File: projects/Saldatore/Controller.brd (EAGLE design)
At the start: 50.8 x 33 mm, 20 parts, among them U1 ATTINY85-P

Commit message: in lavoro saldatore.
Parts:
- R4: value 47-2W -> 120-5W
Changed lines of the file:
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@@
 <drawing>
 <settings>
-<setting alwaysvectorfont="yes"/>
+<setting alwaysvectorfont="no"/>
 <setting verticaltext="up"/>
 </settings>
@@
 <attribute name="VALUE" x="32.29" y="22.99" size="1.27" layer="27" rot="R90"/>
 </element>
-<element name="R4" library="rcl" library_urn="urn:adsk.eagle:library:334" package="0204/7" package3d_urn="urn:adsk.eagle:package:23498/2" value="47-2W" x="36.83" y="44.45" smashed="yes" rot="R270">
+<element name="R4" library="rcl" library_urn="urn:adsk.eagle:library:334" package="0204/7" package3d_urn="urn:adsk.eagle:package:23498/2" value="120-5W" x="36.83" y="44.45" smashed="yes" rot="R270">
 <attribute name="NAME" x="38.1254" y="46.99" size="0.9906" layer="25" ratio="10" rot="R270"/>
 <attribute name="POPULARITY" value="79" x="-8.89" y="6.35" size="1.778" layer="27" rot="R270" display="off"/>

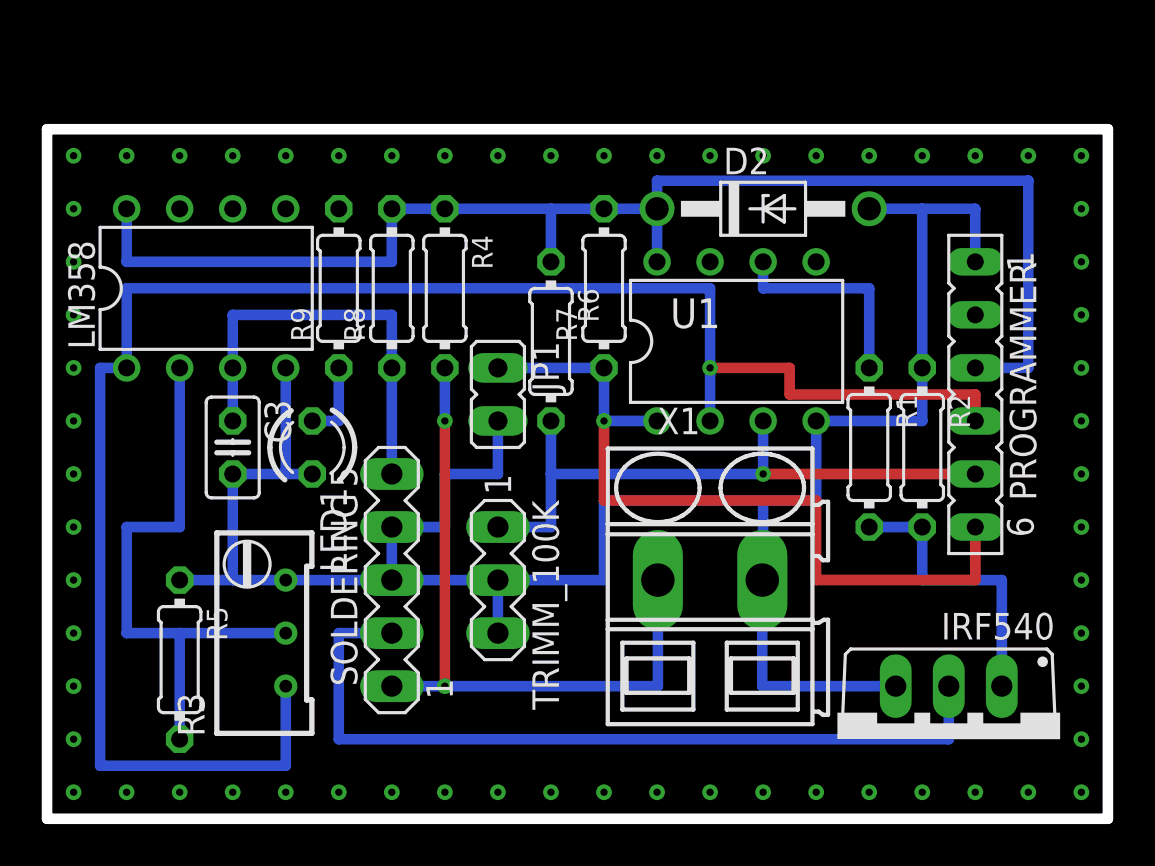
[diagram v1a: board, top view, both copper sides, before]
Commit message: aggiornato saldatore.
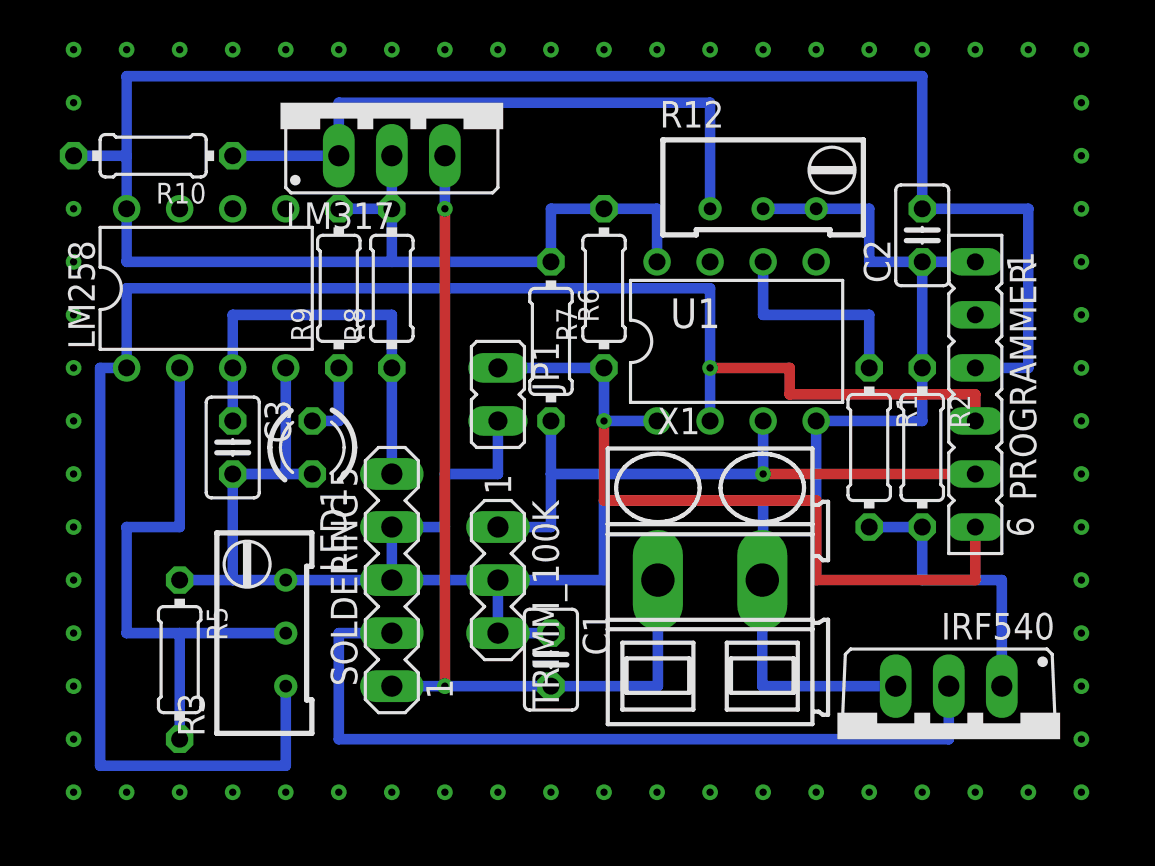
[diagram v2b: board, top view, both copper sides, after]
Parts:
- removed D2: 5v1-1W, diode_MOD:DO41Z10
- removed R4: 120-5W, rcl:0204/7
- added C1: 0.1u, rcl:C025-025X050
- added C2: 1u, rcl:C025-025X050
- added LM317: (no value), v-reg:317TS
- added R10: 240, rcl:0204/7
- added R12: 1k, rcl:RTRIM64W
- R1: value 270 -> 220
- R8: value 10K -> 1k
- renumbered LM358 to LM258
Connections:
- new net N$67: LM317.1, R10.1, R12.1
- net 24V: now also C1.2, LM317.3; no longer R4.2
- net GND: now also C1.1, C2.1, R12.2, R12.3; no longer D2.A
- net VCC: now also C2.2, LM317.2, R10.2; no longer D2.C, R4.1
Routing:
- net VCC: track 66.2 -> 109.2 mm
- net N$67: track 0.00 -> 30.5 mm
- net 24V: track 33.1 -> 43.2 mm
- net GND: track 105.5 -> 110.6 mm
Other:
- board outline removed

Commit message: in lavoro immagine scheda controller.
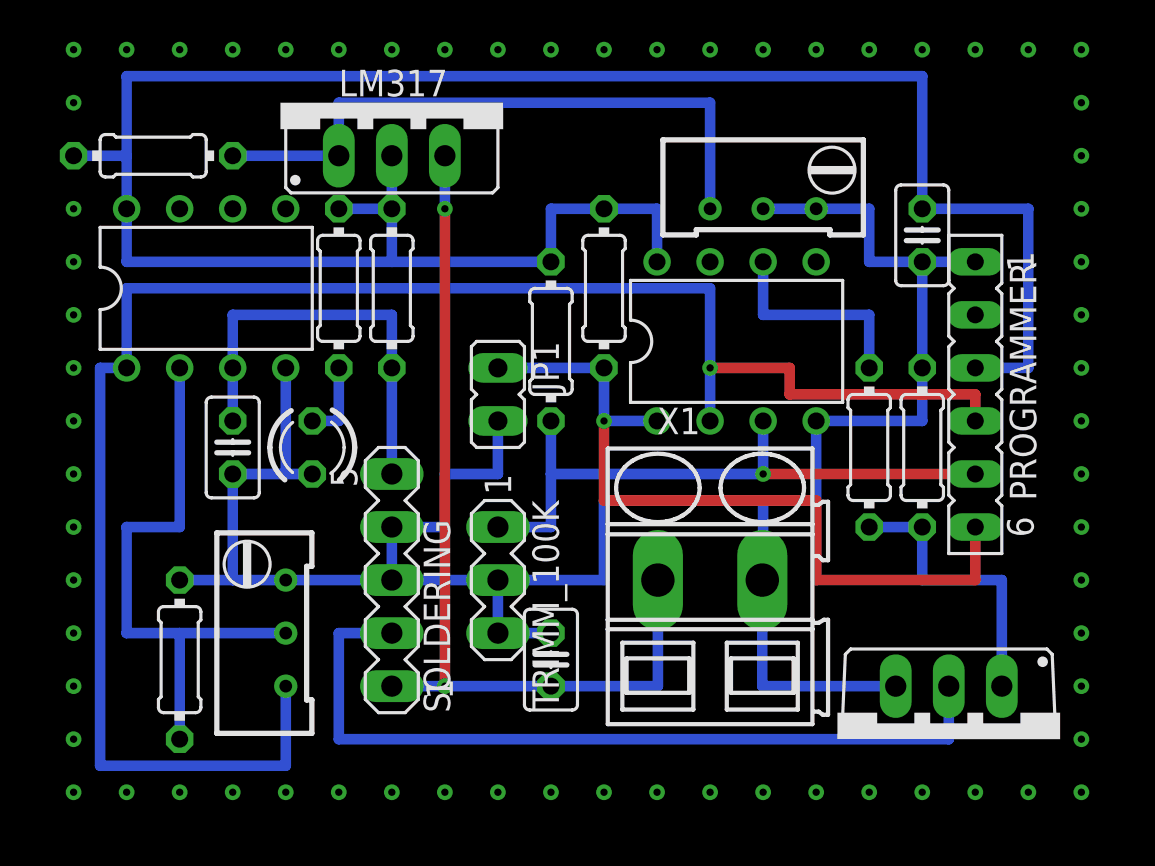
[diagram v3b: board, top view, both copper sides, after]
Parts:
- LM258: value LM358N -> LM258N
